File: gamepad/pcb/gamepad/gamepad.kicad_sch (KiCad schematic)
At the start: 9 parts, among them U3 RP2040-ZERO

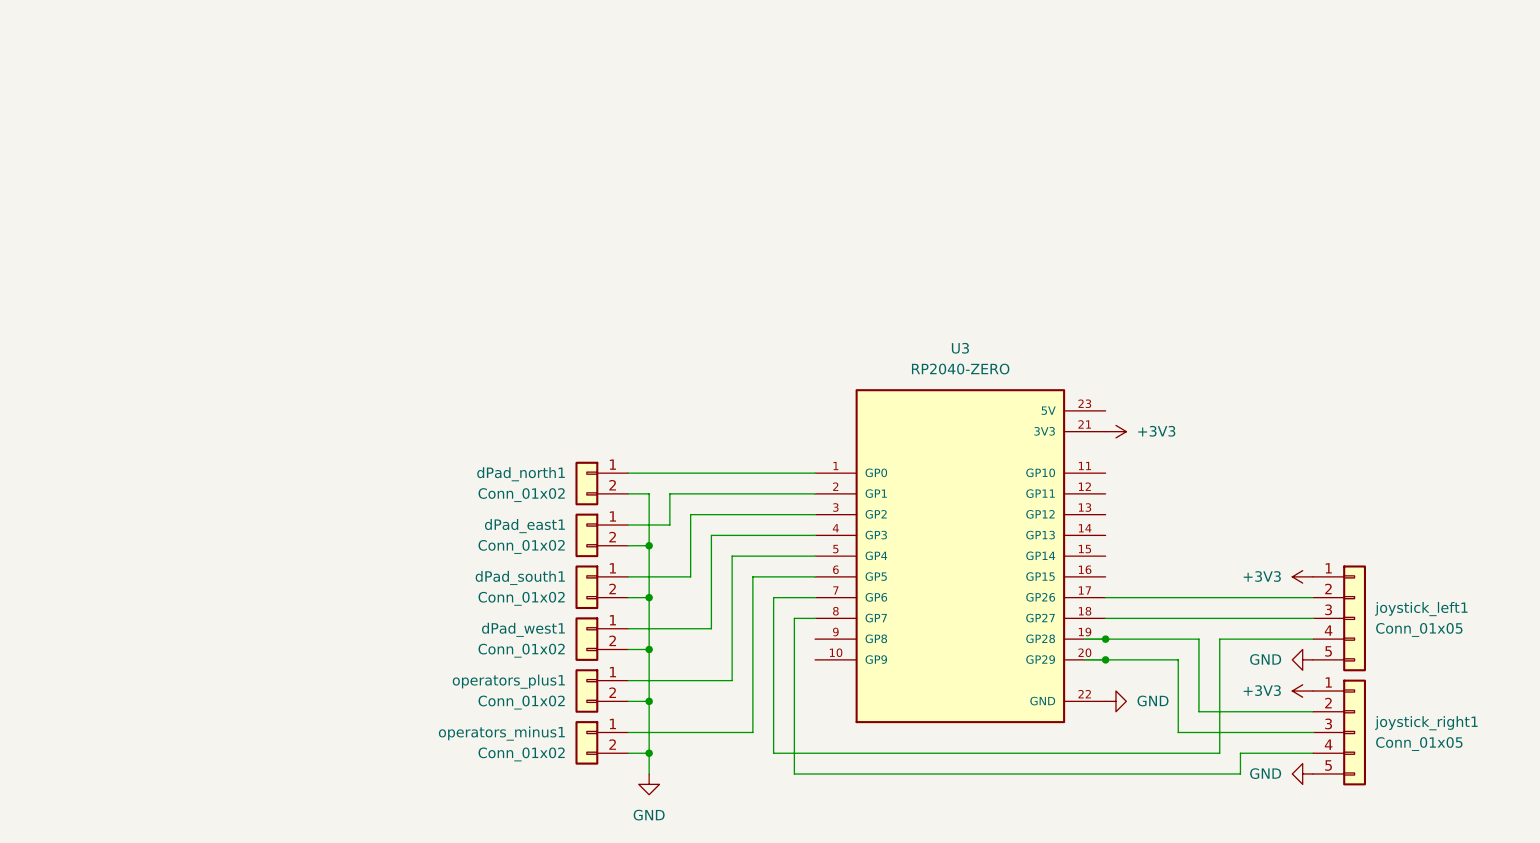
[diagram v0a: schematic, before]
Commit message: upt: pcb
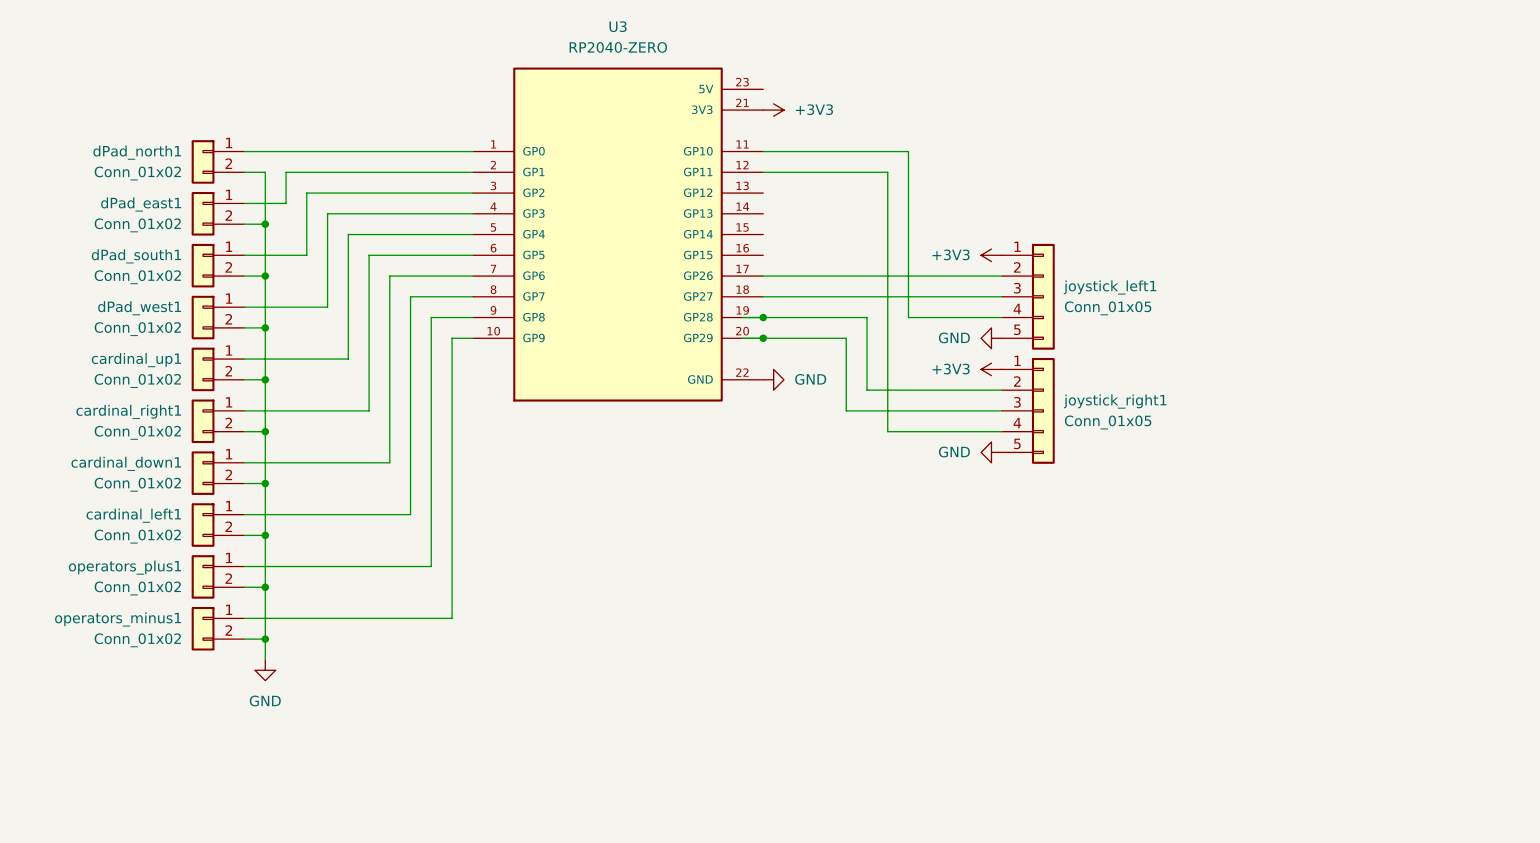
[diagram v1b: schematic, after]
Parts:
- added cardinal_down1, cardinal_left1, cardinal_right1, cardinal_up1: Conn_01x02, Connector_JST:JST_XH_B2B-XH-A_1x02_P2.50mm_Vertical, symbol Connector_Generic:Conn_01x02
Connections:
- net GND: now also cardinal_down1.2 (Pin_2), cardinal_left1.2 (Pin_2), cardinal_right1.2 (Pin_2), cardinal_up1.2 (Pin_2)
- net at operators_plus1.1 (Pin_1): now also U3.9 (GP8); no longer U3.5 (GP4)
- net at U3.10 (GP9): now also operators_minus1.1 (Pin_1)
- net at U3.11 (GP10): now also joystick_left1.4 (Pin_4)
- net at U3.12 (GP11): now also joystick_right1.4 (Pin_4)
- net at U3.6 (GP5): now also cardinal_right1.1 (Pin_1); no longer operators_minus1.1 (Pin_1)
- net at U3.7 (GP6): now also cardinal_down1.1 (Pin_1); no longer joystick_left1.4 (Pin_4)
- net at U3.8 (GP7): now also cardinal_left1.1 (Pin_1); no longer joystick_right1.4 (Pin_4)
- new net: U3.5 (GP4), cardinal_up1.1 (Pin_1)
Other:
- moved on the sheet: U3, dPad_east1, dPad_north1, dPad_south1, dPad_west1, joystick_left1, joystick_right1, operators_minus1, operators_plus1
